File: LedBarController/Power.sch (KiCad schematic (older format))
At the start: 24 parts, among them J1201 Barrel_Jack_Switch, Q1201 FQP47P06, U1201 AMS1117-5.0, U1202 INA219AxD

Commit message: Reduced circuit by remove extra features. Routed whole board. Needs refinement
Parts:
- D1202: footprint LED_THT:LED_D3.0mm -> LED_SMD:LED_0805_2012Metric_Pad1.15x1.40mm_HandSolder
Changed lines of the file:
@@
 $Descr A4 11693 8268
 encoding utf-8
-Sheet 12 14
+Sheet 11 13
 Title ""
 Date ""
@@
 F 0 "D1202" V 9539 4132 50  0000 R CNN
 F 1 "Blue" V 9448 4132 50  0000 R CNN
-F 2 "LED_THT:LED_D3.0mm" H 9500 4250 50  0001 C CNN
+F 2 "LED_SMD:LED_0805_2012Metric_Pad1.15x1.40mm_HandSolder" H 9500 4250 50  0001 C CNN
 F 3 "~" H 9500 4250 50  0001 C CNN
 F 4 "POWER" H 9500 4250 50  0001 C CNN "Feature"

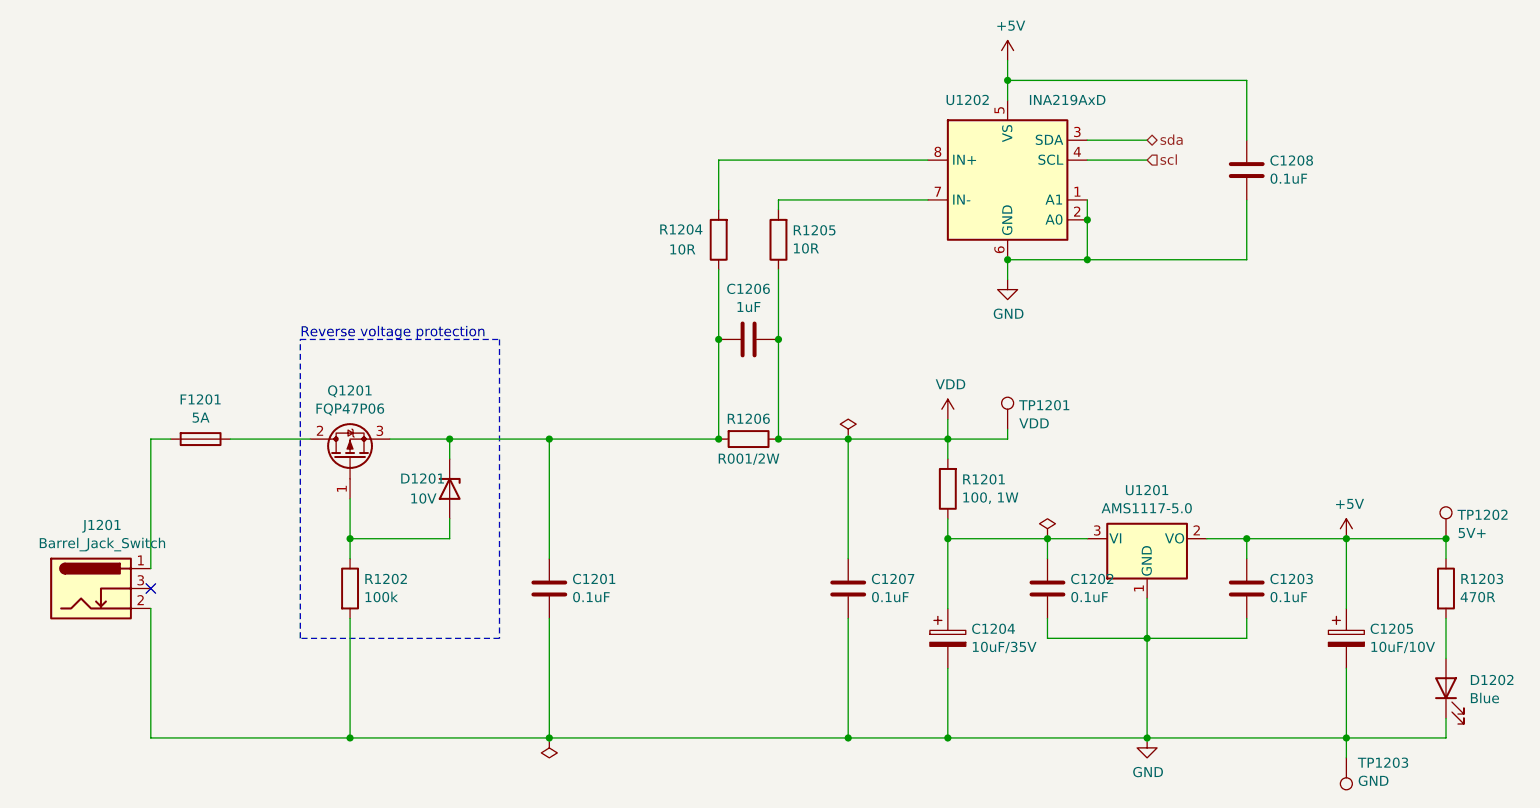
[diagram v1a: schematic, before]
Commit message: Added surge protection
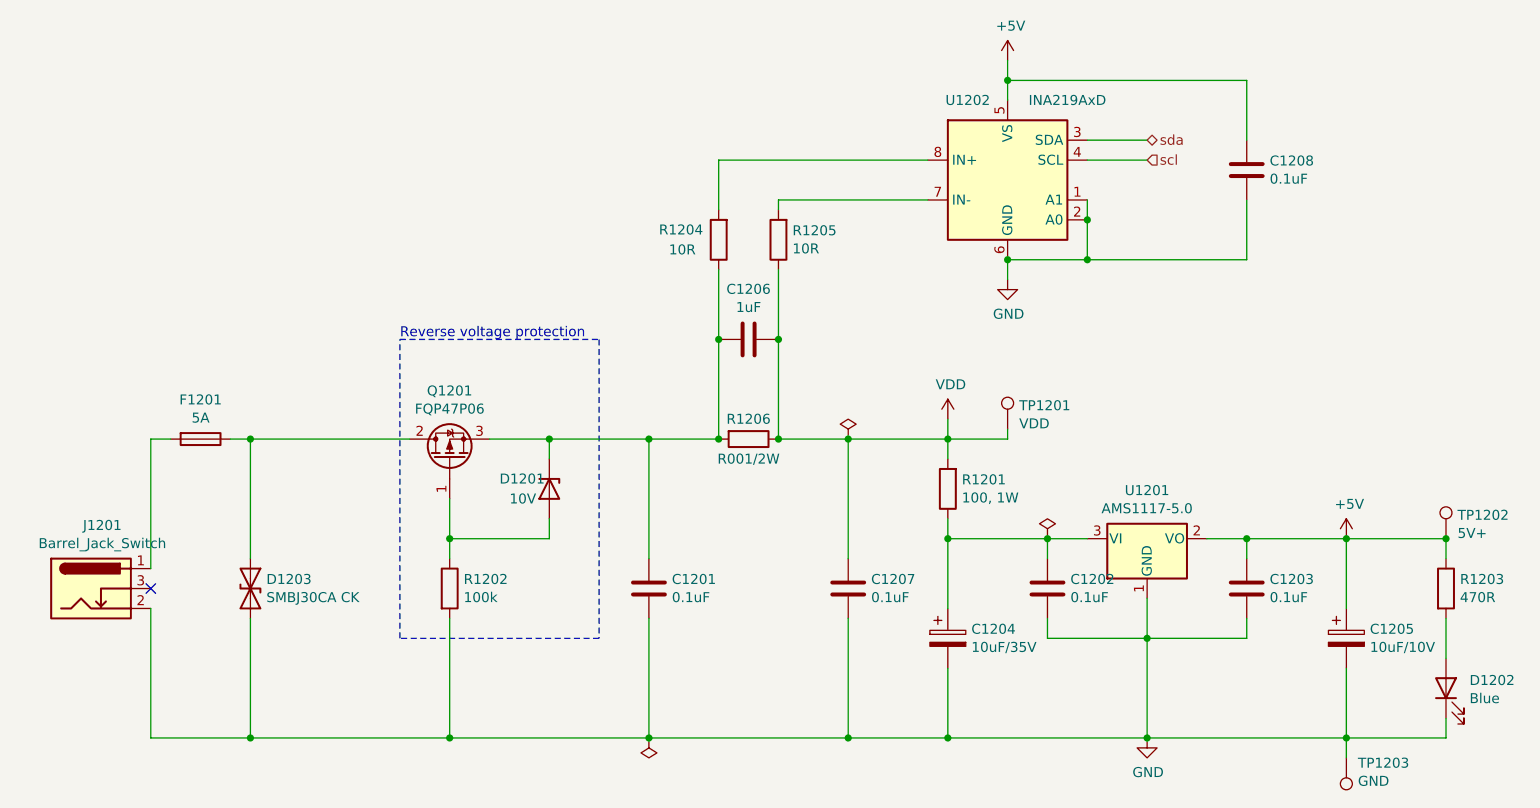
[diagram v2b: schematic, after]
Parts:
- added D1203: SMBJ30CA CK, Diode_SMD:D_SMB_Handsoldering, symbol Device:D_TVS
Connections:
- net GND: now also D1203.2 (A2)
- net at F1201.1, Q1201.2 (D): now also D1203.1 (A1)
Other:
- moved on the sheet: C1201, D1201, Q1201, R1202
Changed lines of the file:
@@
 L Device:C C1201
 U 1 1 5F7F8388
-P 5000 3750
-F 0 "C1201" H 5115 3796 50  0000 L CNN
-F 1 "0.1uF" H 5115 3705 50  0000 L CNN
-F 2 "Capacitor_SMD:C_0805_2012Metric_Pad1.18x1.45mm_HandSolder" H 5038 3600 50  0001 C CNN
-F 3 "~" H 5000 3750 50  0001 C CNN
-F 4 "POWER" H 5000 3750 50  0001 C CNN "Feature"
-F 5 "0.0057" H 5000 3750 50  0001 C CNN "Price"
-F 6 "yes" H 5000 3750 50  0001 C CNN "is stock"
-	1    5000 3750
+P 5500 3750
+F 0 "C1201" H 5615 3796 50  0000 L CNN
+F 1 "0.1uF" H 5615 3705 50  0000 L CNN
+F 2 "Capacitor_SMD:C_0805_2012Metric_Pad1.18x1.45mm_HandSolder" H 5538 3600 50  0001 C CNN
+F 3 "~" H 5500 3750 50  0001 C CNN
+F 4 "POWER" H 5500 3750 50  0001 C CNN "Feature"
+F 5 "0.0057" H 5500 3750 50  0001 C CNN "Price"
+F 6 "yes" H 5500 3750 50  0001 C CNN "is stock"
+	1    5500 3750
 	1    0    0    -1
 $EndComp
@@
 Wire Wire Line
 	7000 3000 7000 3100
-Wire Wire Line
-	5000 3000 5000 3600
-Connection ~ 5000 3000
-Wire Wire Line
-	5000 3900 5000 4500
-Connection ~ 5000 4500
 $Comp
 L power:PWR_FLAG #FLG01203
 U 1 1 5F820B2B
-P 5000 4500
-F 0 "#FLG01203" H 5000 4575 50  0001 C CNN
-F 1 "PWR_FLAG" H 5000 4673 50  0001 C CNN
-F 2 "" H 5000 4500 50  0001 C CNN
-F 3 "~" H 5000 4500 50  0001 C CNN
-	1    5000 4500
+P 5500 4500
+F 0 "#FLG01203" H 5500 4575 50  0001 C CNN
+F 1 "PWR_FLAG" H 5500 4673 50  0001 C CNN
+F 2 "" H 5500 4500 50  0001 C CNN
+F 3 "~" H 5500 4500 50  0001 C CNN
+	1    5500 4500
 	-1   0    0    1
 $EndComp
@@
 L Device:Q_PMOS_GDS Q1201
 U 1 1 5FA735DA
-P 4000 3100
-F 0 "Q1201" V 4342 3100 50  0000 C CNN
-F 1 "FQP47P06" V 4251 3100 50  0000 C CNN
-F 2 "Package_TO_SOT_THT:TO-220-3_Vertical" H 4200 3200 50  0001 C CNN
-F 3 "~" H 4000 3100 50  0001 C CNN
-F 4 "REVERSEPOLARITY_SUPPORTED" H 4000 3100 50  0001 C CNN "Feature"
-F 5 "0.386" H 4000 3100 50  0001 C CNN "Price"
-F 6 "no" H 4000 3100 50  0001 C CNN "is stock"
-	1    4000 3100
+P 4500 3100
+F 0 "Q1201" V 4842 3100 50  0000 C CNN
+F 1 "FQP47P06" V 4751 3100 50  0000 C CNN
+F 2 "Package_TO_SOT_THT:TO-220-3_Vertical" H 4700 3200 50  0001 C CNN
+F 3 "~" H 4500 3100 50  0001 C CNN
+F 4 "REVERSEPOLARITY_SUPPORTED" H 4500 3100 50  0001 C CNN "Feature"
+F 5 "0.386" H 4500 3100 50  0001 C CNN "Price"
+F 6 "no" H 4500 3100 50  0001 C CNN "is stock"
+	1    4500 3100
 	0    -1   -1   0
 $EndComp
 Wire Wire Line
-	3400 3000 3800 3000
-Wire Wire Line
-	3000 4500 4000 4500
+	3500 4500 4500 4500
 $Comp
 L Device:D_Zener D1201
 U 1 1 5FA7B9A0
-P 4500 3250
-F 0 "D1201" V 4450 3000 50  0000 L CNN
-F 1 "10V" V 4550 3050 50  0000 L CNN
-F 2 "Diode_SMD:D_1206_3216Metric_Pad1.42x1.75mm_HandSolder" H 4500 3250 50  0001 C CNN
-F 3 "~" H 4500 3250 50  0001 C CNN
-F 4 "REVERSEPOLARITY_SUPPORTED" H 4500 3250 50  0001 C CNN "Feature"
-F 5 "0.0073" H 4500 3250 50  0001 C CNN "Price"
-F 6 "yes" H 4500 3250 50  0001 C CNN "is stock"
-	1    4500 3250
+P 5000 3250
+F 0 "D1201" V 4950 3000 50  0000 L CNN
+F 1 "10V" V 5050 3050 50  0000 L CNN
+F 2 "Diode_SMD:D_1206_3216Metric_Pad1.42x1.75mm_HandSolder" H 5000 3250 50  0001 C CNN
+F 3 "~" H 5000 3250 50  0001 C CNN
+F 4 "REVERSEPOLARITY_SUPPORTED" H 5000 3250 50  0001 C CNN "Feature"
+F 5 "0.0073" H 5000 3250 50  0001 C CNN "Price"
+F 6 "yes" H 5000 3250 50  0001 C CNN "is stock"
+	1    5000 3250
 	0    1    1    0
 $EndComp
@@
 L Device:R R1202
 U 1 1 5FA7CE6E
-P 4000 3750
-F 0 "R1202" H 4070 3796 50  0000 L CNN
-F 1 "100k" H 4070 3705 50  0000 L CNN
-F 2 "Resistor_SMD:R_0805_2012Metric_Pad1.20x1.40mm_HandSolder" V 3930 3750 50  0001 C CNN
-F 3 "~" H 4000 3750 50  0001 C CNN
-F 4 "REVERSEPOLARITY_SUPPORTED" H 4000 3750 50  0001 C CNN "Feature"
-F 5 "0.0036" H 4000 3750 50  0001 C CNN "Price"
-F 6 "yes" H 4000 3750 50  0001 C CNN "is stock"
-	1    4000 3750
-	1    0    0    -1
-$EndComp
-Wire Wire Line
-	4200 3000 4500 3000
-Wire Wire Line
-	4500 3100 4500 3000
-Connection ~ 4500 3000
-Wire Wire Line
-	4500 3000 5000 3000
-Wire Wire Line
-	4500 3400 4500 3500
-Wire Wire Line
-	4500 3500 4000 3500
-Wire Wire Line
-	4000 3500 4000 3300
-Wire Wire Line
-	4000 3500 4000 3600
-Connection ~ 4000 3500
-Wire Wire Line
-	4000 3900 4000 4500
-Connection ~ 4000 4500
-Wire Wire Line
-	4000 4500 5000 4500
+P 4500 3750
+F 0 "R1202" H 4570 3796 50  0000 L CNN
+F 1 "100k" H 4570 3705 50  0000 L CNN
+F 2 "Resistor_SMD:R_0805_2012Metric_Pad1.20x1.40mm_HandSolder" V 4430 3750 50  0001 C CNN
+F 3 "~" H 4500 3750 50  0001 C CNN
+F 4 "REVERSEPOLARITY_SUPPORTED" H 4500 3750 50  0001 C CNN "Feature"
+F 5 "0.0036" H 4500 3750 50  0001 C CNN "Price"
+F 6 "yes" H 4500 3750 50  0001 C CNN "is stock"
+	1    4500 3750
+	1    0    0    -1
+$EndComp
+Wire Wire Line
+	4700 3000 5000 3000
+Wire Wire Line
+	5000 3100 5000 3000
+Wire Wire Line
+	5000 3400 5000 3500
+Wire Wire Line
+	5000 3500 4500 3500
+Wire Wire Line
+	4500 3500 4500 3300
+Wire Wire Line
+	4500 3500 4500 3600
+Connection ~ 4500 3500
+Wire Wire Line
+	4500 3900 4500 4500
+Connection ~ 4500 4500
+Wire Wire Line
+	4500 4500 5500 4500
 Wire Notes Line
-	3750 2500 4750 2500
+	4250 2500 5250 2500
 Wire Notes Line
-	4750 2500 4750 4000
+	5250 2500 5250 4000
 Wire Notes Line
-	4750 4000 3750 4000
+	5250 4000 4250 4000
 Wire Notes Line
-	3750 4000 3750 2500
-Text Notes 3750 2500 0    50   ~ 0
+	4250 4000 4250 2500
+Text Notes 4250 2500 0    50   ~ 0
 Reverse voltage protection
 Wire Wire Line
@@
 Wire Wire Line
 	5850 1600 6900 1600
-Wire Wire Line
-	5000 3000 5850 3000
 Connection ~ 5850 3000
 Wire Wire Line
@@
 Text HLabel 8000 1600 2    50   Input ~ 0
 scl
-Wire Wire Line
-	5000 4500 6500 4500
 $Comp
 L Device:C C1207
@@
 Wire Wire Line
 	8500 1800 8500 2100
+$Comp
+L Device:D_TVS D1203
+U 1 1 5FC9A3E5
+P 3500 3750
+F 0 "D1203" V 3454 3830 50  0000 L CNN
+F 1 "SMBJ30CA CK" V 3545 3830 50  0000 L CNN
+F 2 "Diode_SMD:D_SMB_Handsoldering" H 3500 3750 50  0001 C CNN
+F 3 "~" H 3500 3750 50  0001 C CNN
+	1    3500 3750
+	0    1    1    0
+$EndComp
+Wire Wire Line
+	5500 3600 5500 3000
+Wire Wire Line
+	5500 3000 5850 3000
+Wire Wire Line
+	5500 3900 5500 4500
+Wire Wire Line
+	5500 4500 6500 4500
+Connection ~ 5500 4500
+Wire Wire Line
+	5000 3000 5500 3000
+Connection ~ 5000 3000
+Connection ~ 5500 3000
+Wire Wire Line
+	3400 3000 3500 3000
+Wire Wire Line
+	3000 4500 3500 4500
+Wire Wire Line
+	3500 4500 3500 3900
+Connection ~ 3500 4500
+Wire Wire Line
+	3500 3600 3500 3000
+Connection ~ 3500 3000
+Wire Wire Line
+	3500 3000 4300 3000
 $EndSCHEMATC
